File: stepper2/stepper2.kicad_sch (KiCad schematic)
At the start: 20 parts, among them J1 DB25_Socket, J2 Conn_02x10_Odd_Even, J3 DB25_Pins, J4 Conn_02x10_Odd_Even, J5 Blue Pill, J6 IPS 240*240, SW2 SW_Push, SW3 SW_Push, SW4 SW_SPDT, SW5 SW_Push_SPDT

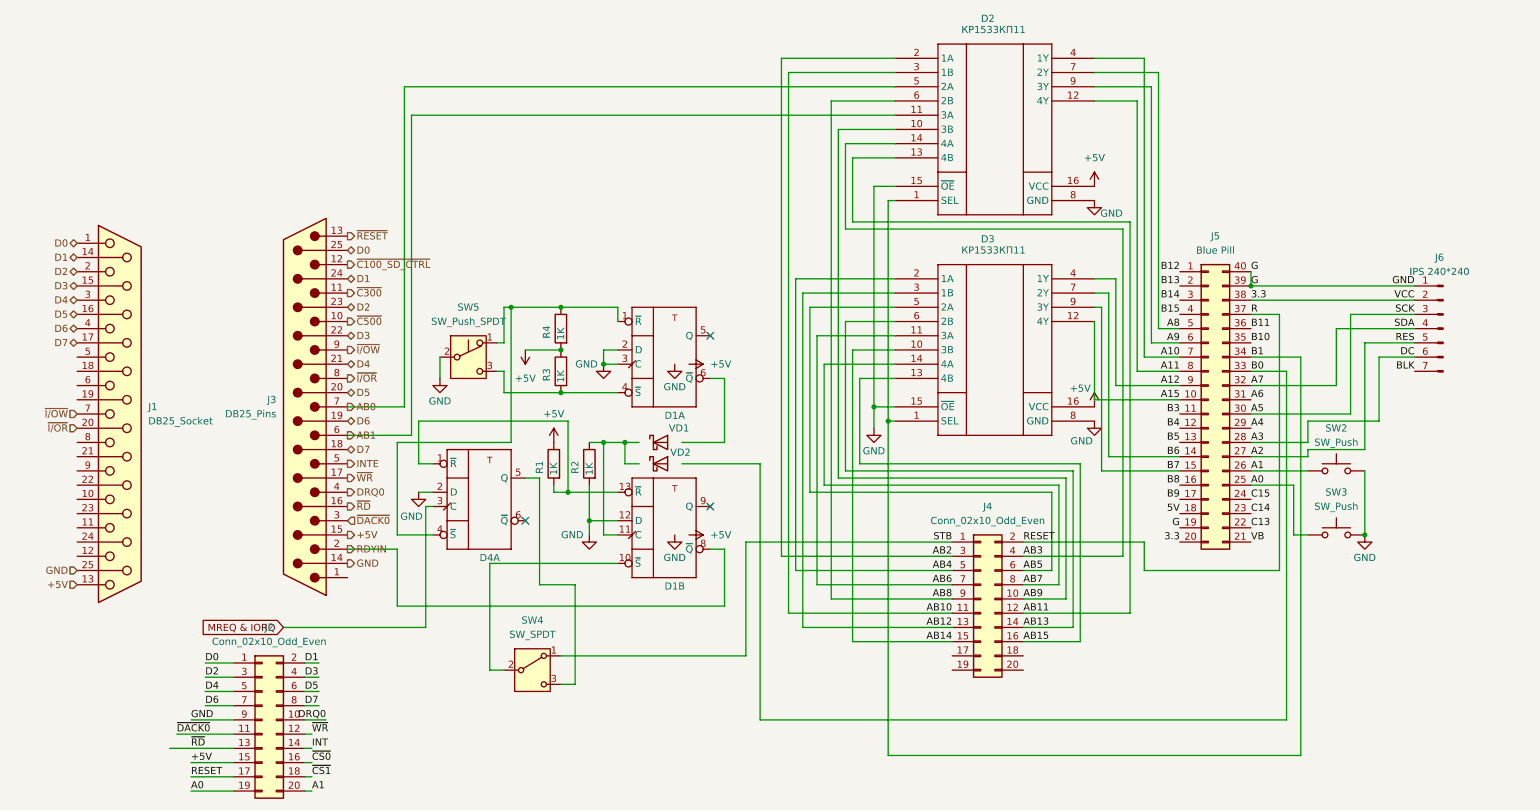
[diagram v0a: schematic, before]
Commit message: Fix schemes
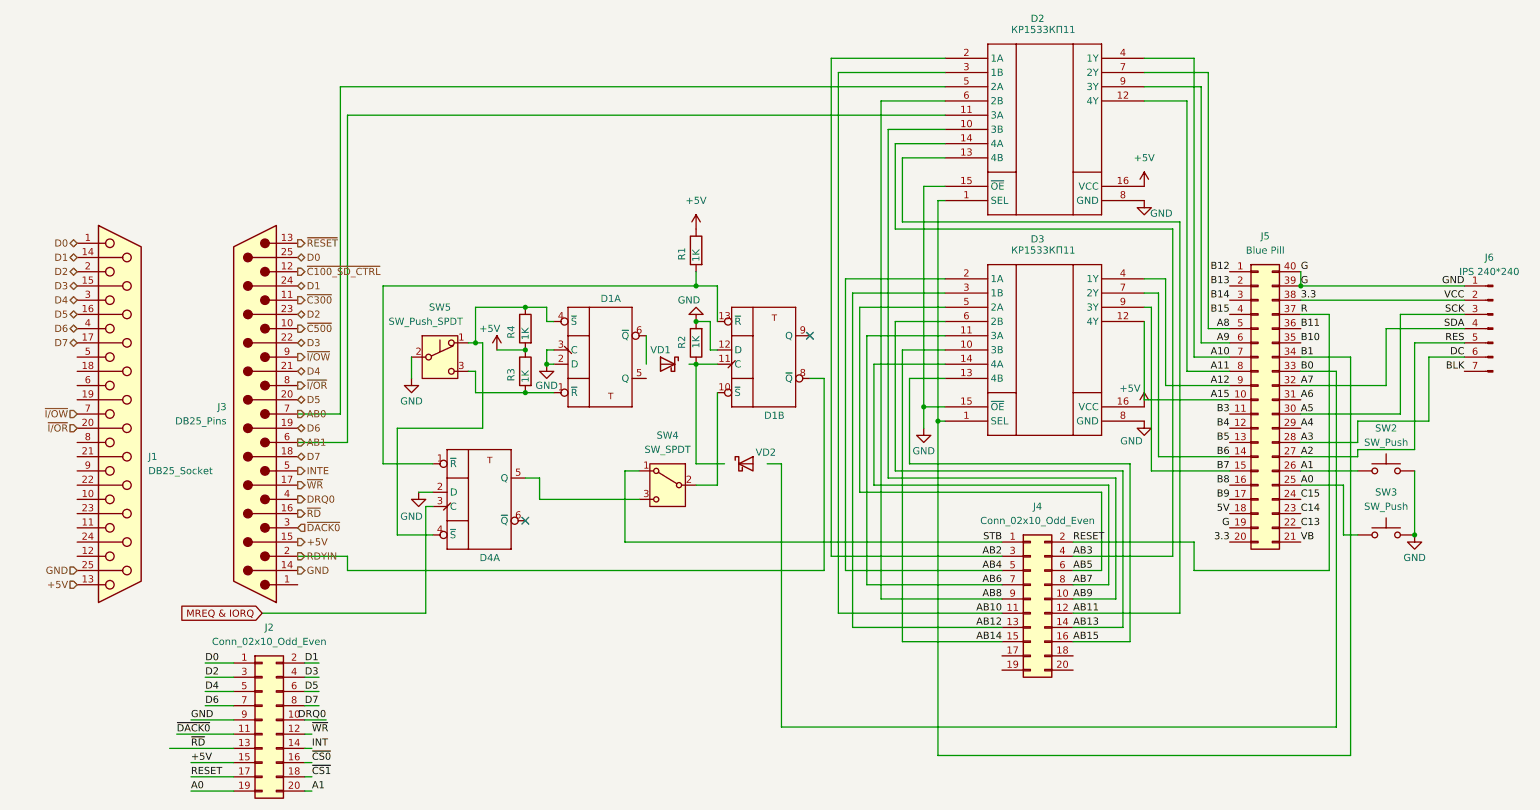
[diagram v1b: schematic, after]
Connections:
- net +5V: no longer D1.14 (VCC), D1.14 (VCC), D4.14 (VCC), J5.20 (Pin_20), J5.38 (Pin_38), J6.2 (Pin_2)
- net at D4.4 (~{S}), R4.1, SW5.1 (A): now also D1.4 (~{S}); no longer D1.1 (~{R})
- net at R3.2, SW5.3 (C): now also D1.1 (~{R}); no longer D1.4 (~{S})
- new net VCC: D1.14 (VCC), D1.14 (VCC), D4.14 (VCC), J5.20 (Pin_20), J5.38 (Pin_38), J6.2 (Pin_2)
- no-connect marks 3 -> 2
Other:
- moved on the sheet: D2, D3, J3, J4, J5, J6, R3, R4, SW2, SW3, SW5, VD2
